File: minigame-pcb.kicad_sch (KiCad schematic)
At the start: 87 parts, among them IC1 HT16K33A-28SSOP, J1 USB_C_Receptacle_USB2.0_16P, U2 AMS1117-3.3, U3 W25Q128JVS

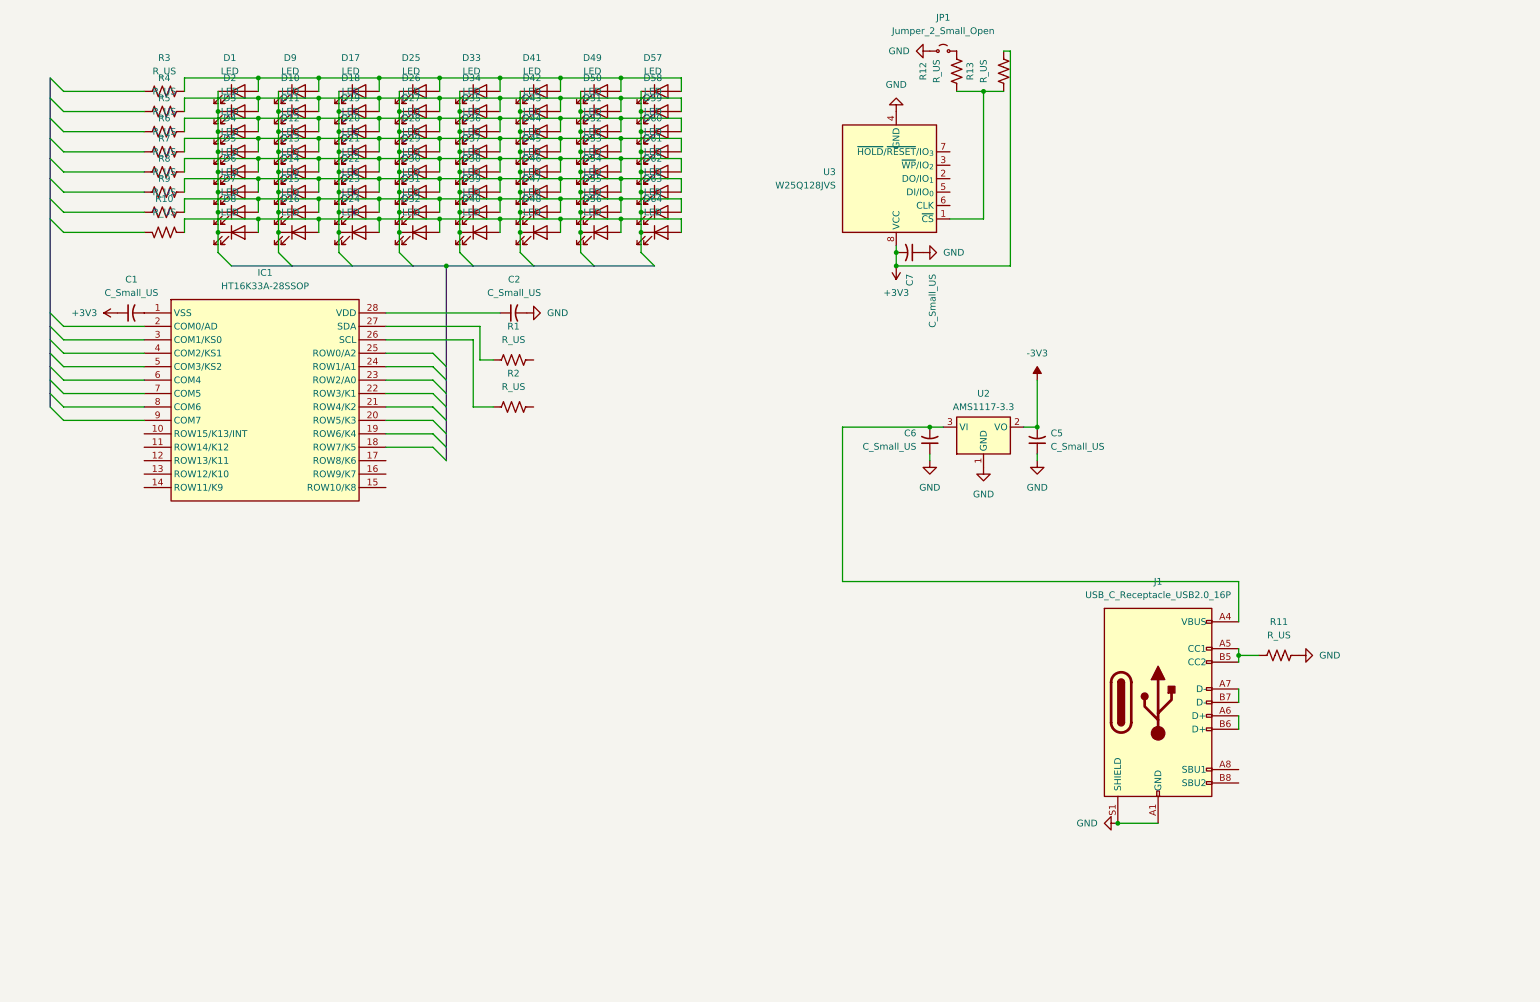
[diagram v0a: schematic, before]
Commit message: e
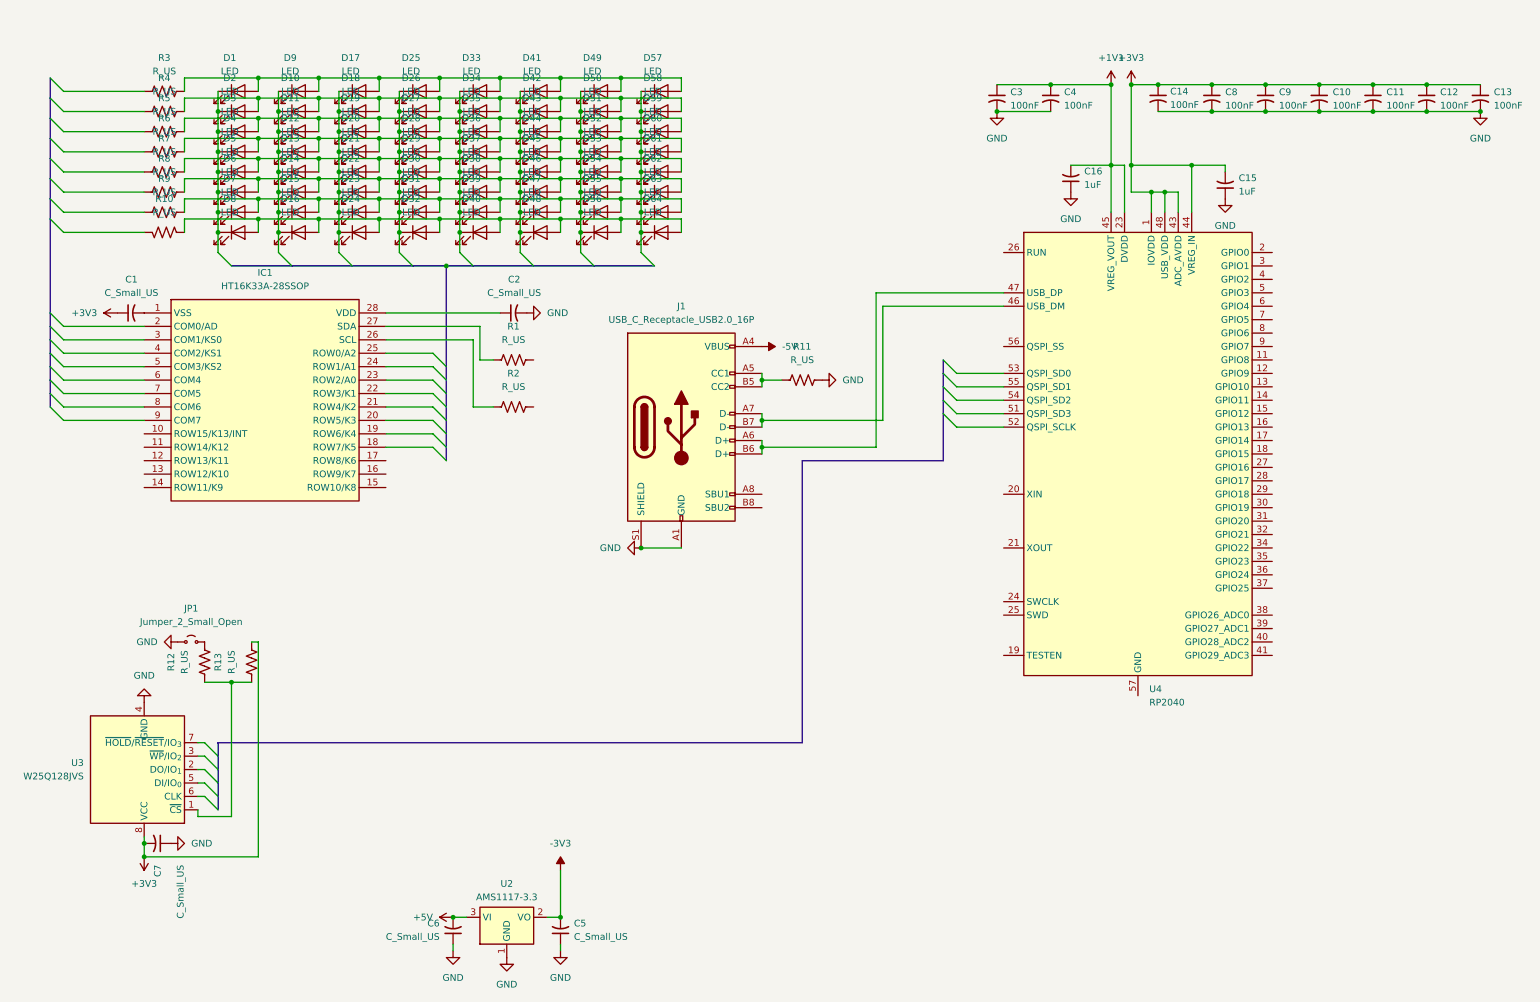
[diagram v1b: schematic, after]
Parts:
- added C10, C11, C12, C13, C14, C3, C4, C8, C9: 100nF, symbol Device:C_Small_US
- added C15, C16: 1uF, symbol Device:C_Small_US
- added U4: RP2040, Package_DFN_QFN:QFN-56-1EP_7x7mm_P0.4mm_EP3.2x3.2mm, symbol MCU_RaspberryPi:RP2040
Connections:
- net +3V3: now also C10.1, C11.1, C12.1, C13.1, C14.1, C15.2, C8.1, C9.1, U4.1 (IOVDD), U4.10 (IOVDD), U4.22 (IOVDD), U4.33 (IOVDD), U4.42 (IOVDD), U4.43 (ADC_AVDD), U4.44 (VREG_IN), U4.48 (USB_VDD), U4.49 (IOVDD)
- net GND: now also C10.2, C11.2, C12.2, C13.2, C14.2, C15.1, C16.1, C3.2, C4.2, C8.2, C9.2
- net -5V: now reaches J1.A4 (VBUS), J1.A9 (VBUS), J1.B4 (VBUS), J1.B9 (VBUS)
- net -5V: no longer C6.2, U2.3 (VI)
- net at J1.A6 (D+), J1.B6 (D+): now also U4.47 (USB_DP)
- net at J1.A7 (D-), J1.B7 (D-): now also U4.46 (USB_DM)
- new net +1V1: C16.2, C3.1, C4.1, U4.23 (DVDD), U4.45 (VREG_VOUT), U4.50 (DVDD)
- new net +5V: C6.2, U2.3 (VI)
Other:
- moved on the sheet: C5, C6, C7, J1, JP1, R11, R12, R13, U2, U3
